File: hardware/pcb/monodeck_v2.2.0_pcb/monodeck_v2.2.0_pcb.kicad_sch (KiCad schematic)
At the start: 12 parts, among them SW1 UP, SW2 DOWN, SW3 LEFT, SW4 RIGHT, SW5 SELECT, SW6 START, SW7 B, SW8 A

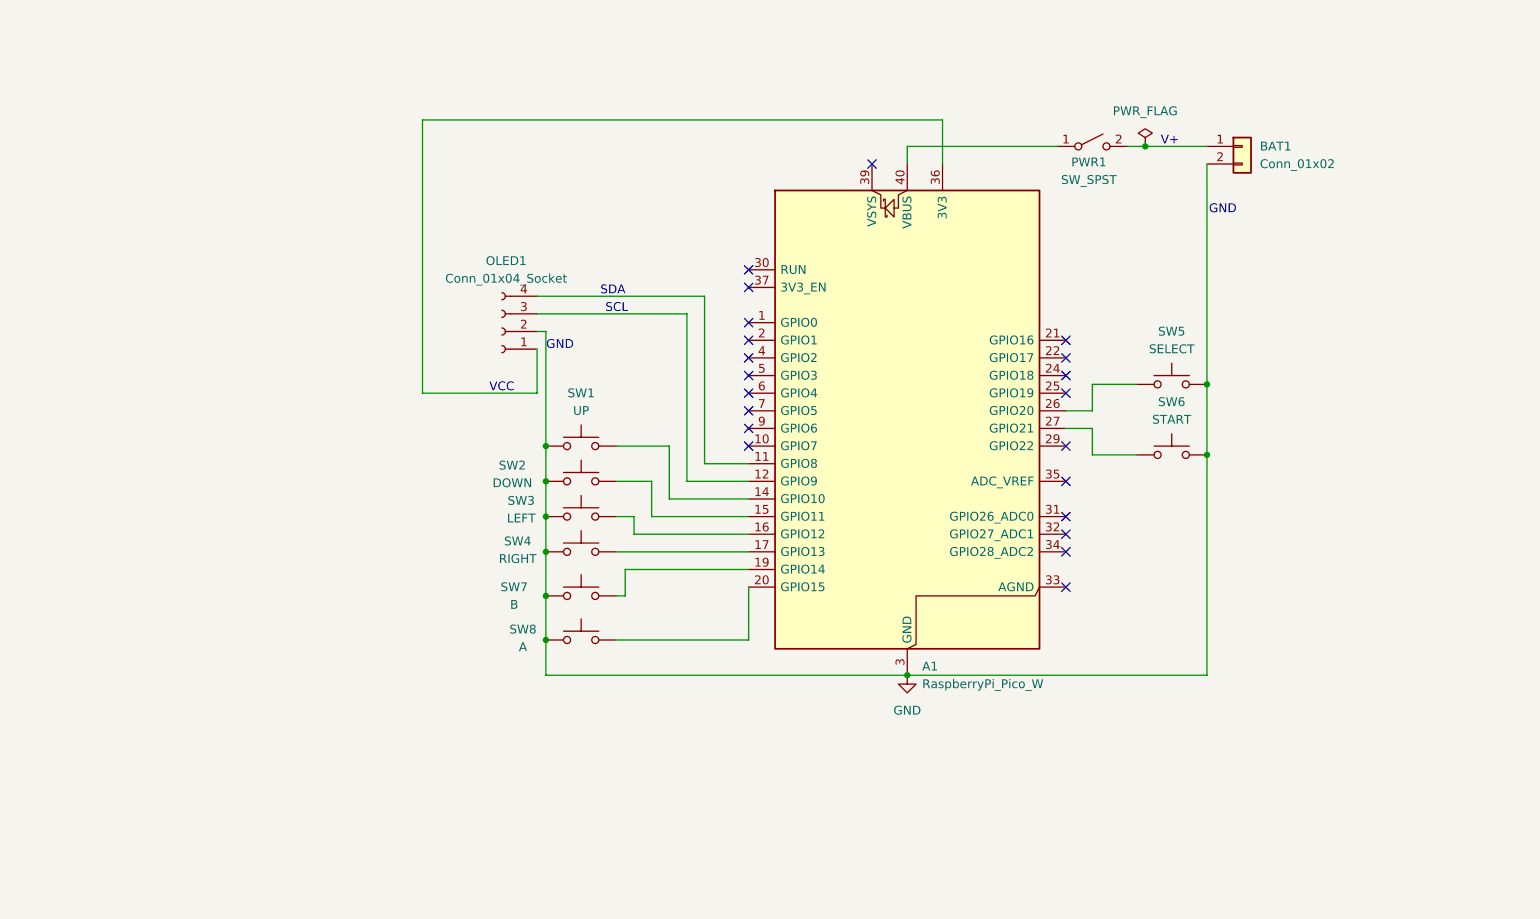
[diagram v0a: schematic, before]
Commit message: updated schematic
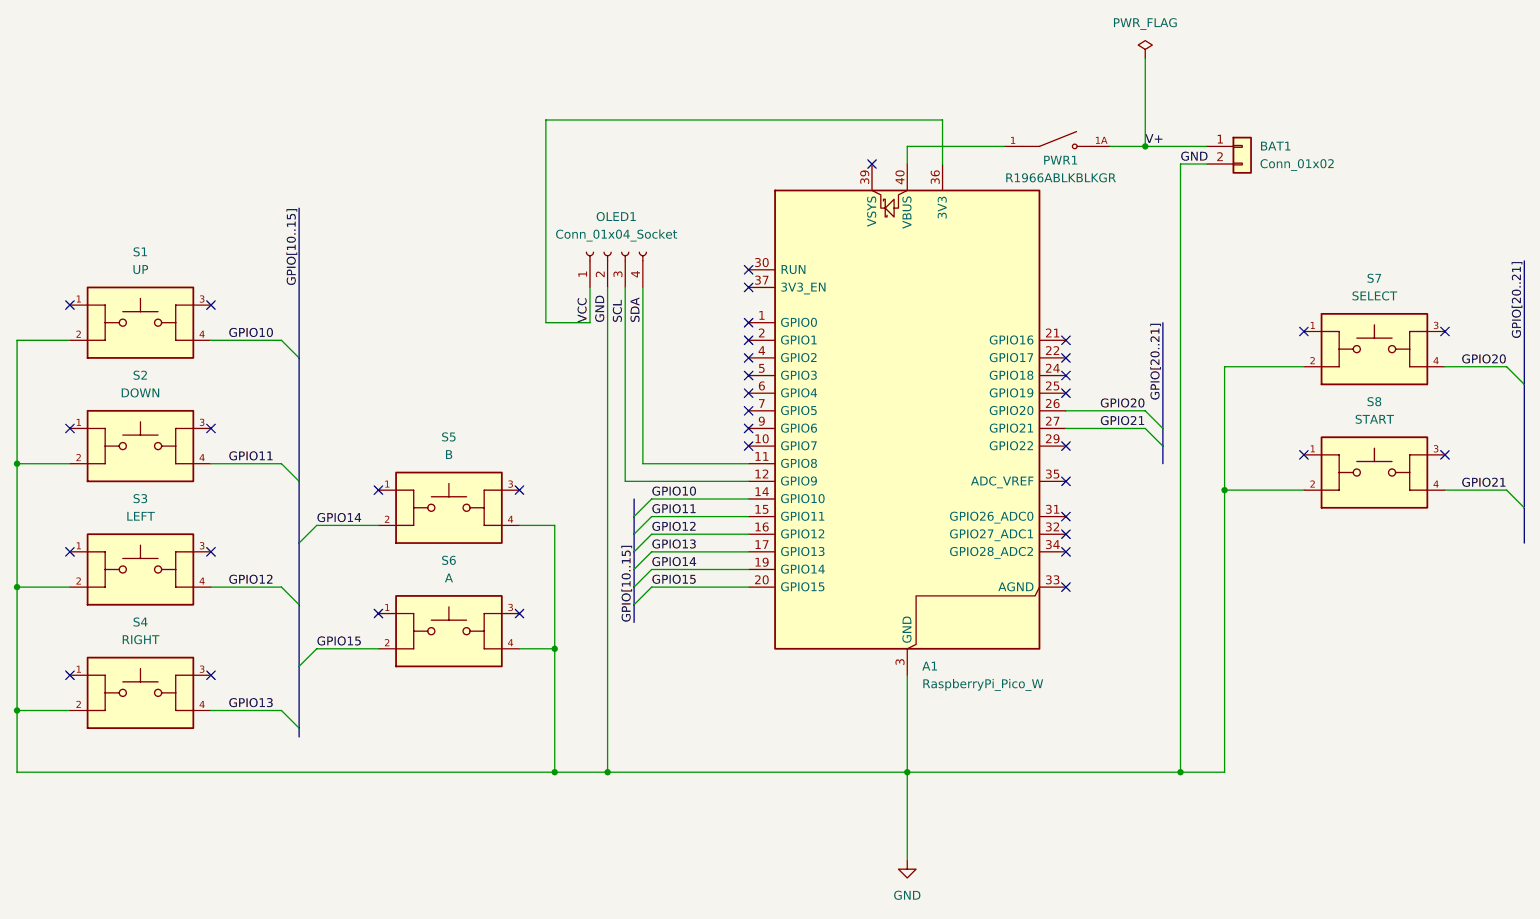
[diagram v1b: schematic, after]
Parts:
- removed PWR1: SW_SPST, symbol Switch:SW_SPST
- removed SW1: UP, symbol Switch:SW_Push
- removed SW2: DOWN, symbol Switch:SW_Push
- removed SW3: LEFT, symbol Switch:SW_Push
- removed SW4: RIGHT, symbol Switch:SW_Push
- removed SW5: SELECT, symbol Switch:SW_Push
- removed SW6: START, symbol Switch:SW_Push
- removed SW7: B, symbol Switch:SW_Push
- removed SW8: A, symbol Switch:SW_Push
- added PWR1: R1966ABLKBLKGR, R1966ABLKBLKGR:SW_R1966ABLKBLKGR, symbol R1966ABLKBLKGR:R1966ABLKBLKGR
- added S1: UP, SWT0211-050010GSA_REVA:SW_SWT0211-050010GSA_REVA, symbol SWT0211-050010GSA_REVA:SWT0211-050010GSA_REVA
- added S2: DOWN, SWT0211-050010GSA_REVA:SW_SWT0211-050010GSA_REVA, symbol SWT0211-050010GSA_REVA:SWT0211-050010GSA_REVA
- added S3: LEFT, SWT0211-050010GSA_REVA:SW_SWT0211-050010GSA_REVA, symbol SWT0211-050010GSA_REVA:SWT0211-050010GSA_REVA
- added S4: RIGHT, SWT0211-050010GSA_REVA:SW_SWT0211-050010GSA_REVA, symbol SWT0211-050010GSA_REVA:SWT0211-050010GSA_REVA
- added S5: B, SWT0211-050010GSA_REVA:SW_SWT0211-050010GSA_REVA, symbol SWT0211-050010GSA_REVA:SWT0211-050010GSA_REVA
- added S6: A, SWT0211-050010GSA_REVA:SW_SWT0211-050010GSA_REVA, symbol SWT0211-050010GSA_REVA:SWT0211-050010GSA_REVA
- added S7: SELECT, SWT0211-050010GSA_REVA:SW_SWT0211-050010GSA_REVA, symbol SWT0211-050010GSA_REVA:SWT0211-050010GSA_REVA
- added S8: START, SWT0211-050010GSA_REVA:SW_SWT0211-050010GSA_REVA, symbol SWT0211-050010GSA_REVA:SWT0211-050010GSA_REVA
- BAT1: footprint (none) -> Connector_JST:JST_PH_B2B-PH-K_1x02_P2.00mm_Vertical
- OLED1: footprint (none) -> Connector_PinSocket_2.54mm:PinSocket_1x04_P2.54mm_Vertical
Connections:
- net GND: now also S1.2, S2.2, S3.2, S4.2, S5.4, S6.4, S7.2, S8.2
- net GPIO11: now reaches A1.15 (GPIO11)
- net GPIO11: now also S2.4
- net VCC: now reaches A1.36 (3V3), OLED1.1 (Pin_1)
- net SCL: now reaches A1.12 (GPIO9), OLED1.3 (Pin_3)
- net SDA: now reaches A1.11 (GPIO8), OLED1.4 (Pin_4)
- net GPIO13: now reaches A1.17 (GPIO13)
- net GPIO13: now also S4.4
- net GPIO21: now reaches A1.27 (GPIO21)
- net GPIO21: now also S8.4
- net at A1.40 (VBUS): now also PWR1.1
- net V+: now reaches BAT1.1 (Pin_1)
- net V+: now also PWR1.1A
- net GPIO10: now reaches A1.14 (GPIO10)
- net GPIO10: now also S1.4
- net GPIO12: now reaches A1.16 (GPIO12)
- net GPIO12: now also S3.4
- net GPIO14: now reaches A1.19 (GPIO14)
- net GPIO14: now also S5.2
- net GPIO15: now reaches A1.20 (GPIO15)
- net GPIO15: now also S6.2
- net GPIO20: now reaches A1.26 (GPIO20)
- net GPIO20: now also S7.4
- no-connect marks 21 -> 37
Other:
- note removed: "GND"
- note removed: "SCL"
- note removed: "SDA"
- note removed: "V+"
- note removed: "VCC"
- title: (none) -> MonoDeck_v2.2.0
- moved on the sheet: OLED1
